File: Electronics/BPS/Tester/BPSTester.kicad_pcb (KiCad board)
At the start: 2 copper layers, 43.2 x 96.5 mm, 27 parts, among them J1 Conn_01x13_Male, J2 Conn_01x02_Male

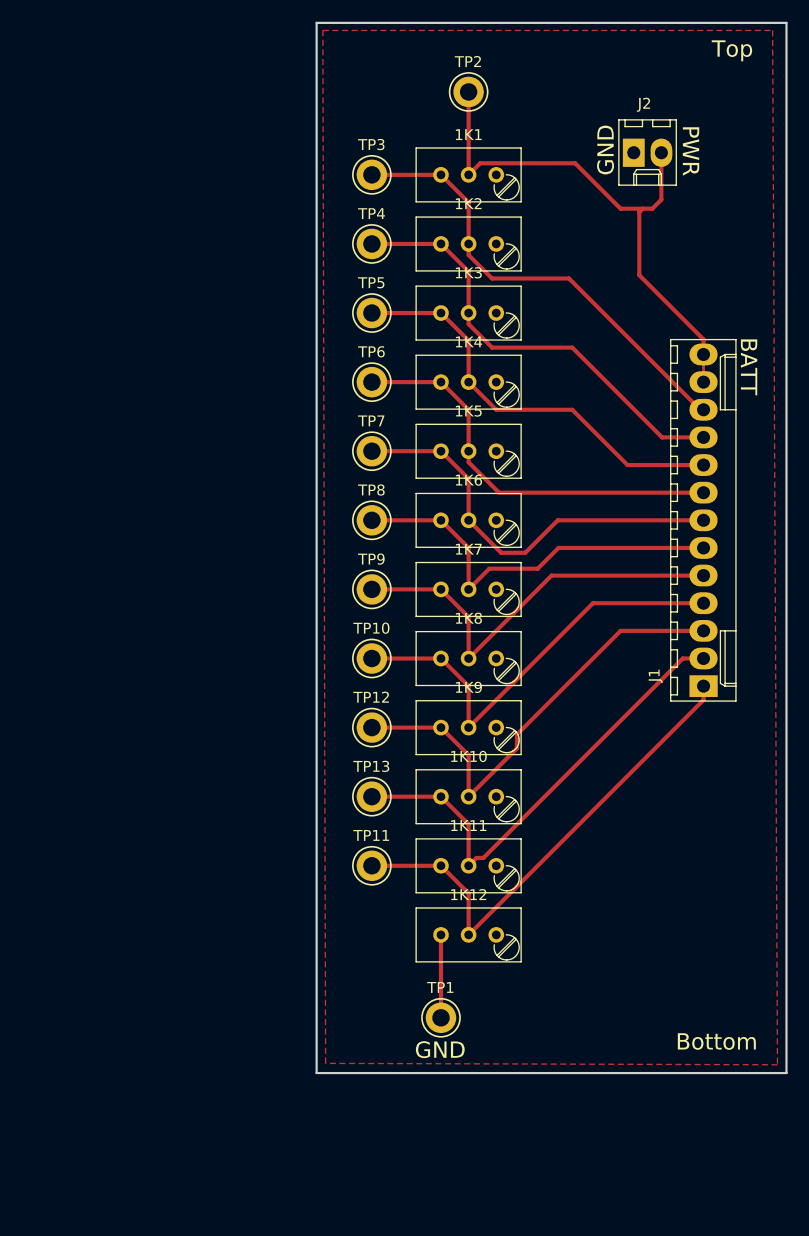
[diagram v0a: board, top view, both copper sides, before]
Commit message: Finalized all boards. Created gerber files.
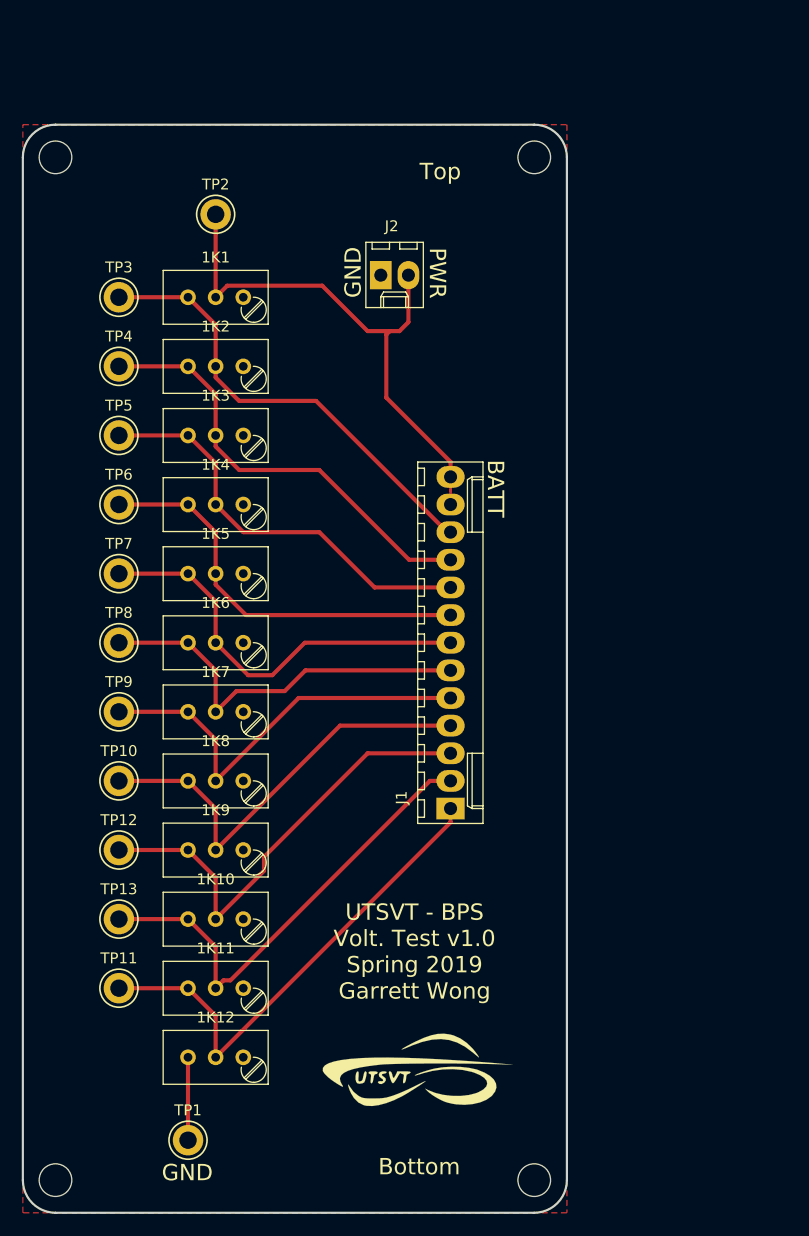
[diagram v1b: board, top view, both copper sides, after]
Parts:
- added G***: LOGO, UTSVT_Special:UTSVT_Logo_Symbol, F.Cu at (136.0, 137.0)
- added REF**: MountingHole_3mm, MountingHole:MountingHole_3mm, F.Cu at (103.0, 147.0)
- added REF**: MountingHole_3mm, MountingHole:MountingHole_3mm, F.Cu at (147.0, 147.0)
- added REF**: MountingHole_3mm, MountingHole:MountingHole_3mm, F.Cu at (147.0, 53.0)
- added REF**: MountingHole_3mm, MountingHole:MountingHole_3mm, F.Cu at (103.0, 53.0)
- moved TP11 25.8 mm to (108.8, 129.4)
- moved TP10 25.8 mm to (108.8, 110.3)
- moved TP12 25.8 mm to (108.8, 116.7)
- moved TP13 25.8 mm to (108.8, 123.0)
- moved TP3 25.8 mm to (108.8, 65.9)
- moved TP4 25.8 mm to (108.8, 72.2)
- moved TP5 25.8 mm to (108.8, 78.6)
- moved TP6 25.8 mm to (108.8, 84.9)
- moved TP7 25.8 mm to (108.8, 91.3)
- moved TP8 25.8 mm to (108.8, 97.6)
- moved TP9 25.8 mm to (108.8, 104.0)
- moved J1 25.8 mm to (139.3, 112.8)
- moved J2 25.8 mm to (132.9, 63.8)
- moved TP1 25.8 mm to (115.2, 143.3)
- moved TP2 25.8 mm to (117.7, 58.2)
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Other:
- board size 43.2 x 96.5 mm -> 50 x 100 mm
- board text added: "Spring 2019: Monolo Alvarez Chase Block Corbin Capo Richard Li Austin Tsao Garrett Wong Sihyung Woo Sijin Woo"
- board text added: "UTSVT - BPS Volt. Test v1.0 Spring 2019 Garrett Wong"
